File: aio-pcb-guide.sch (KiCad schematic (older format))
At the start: 24 parts, among them SW1 SW_Push, U1 ATmega32U4-AU, Y1 16MHz

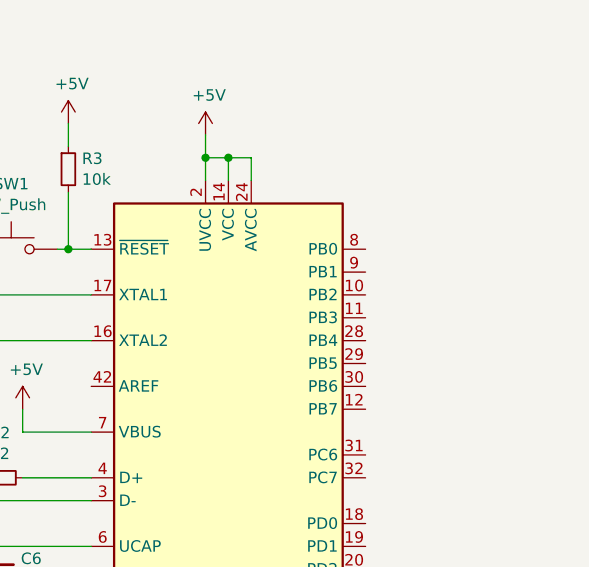
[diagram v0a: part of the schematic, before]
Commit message: Some Routing Completed
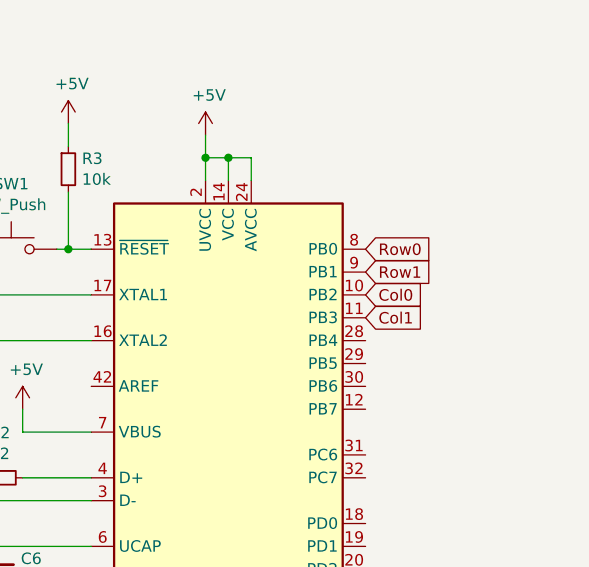
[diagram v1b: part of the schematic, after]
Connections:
- net Col0: now also U1.10 (PB2)
- net Col1: now also U1.11 (PB3)
- net Row0: now also U1.8 (PB0)
- net Row1: now also U1.9 (PB1)
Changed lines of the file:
@@
 EESchema Schematic File Version 4
+LIBS:aio-pcb-guide-cache
 EELAYER 30 0
 EELAYER END
@@
 Wire Notes Line
 	5150 450  5150 3950
+Text GLabel 10350 1550 2    50   Input ~ 0
+Row0
+Text GLabel 10350 1650 2    50   Input ~ 0
+Row1
+Text GLabel 10350 1750 2    50   Input ~ 0
+Col0
+Text GLabel 10350 1850 2    50   Input ~ 0
+Col1
 $EndSCHEMATC
